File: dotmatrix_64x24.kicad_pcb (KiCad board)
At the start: 2 copper layers, 180 x 100 mm, 750 parts, among them CON1 BARREL_JACK, P1 CONN_01X09, P2 CONN_01X09, P3 CONN_01X04, P4 CONN_01X03, P5 USB_OTG, P6 CONN_01X03, Q1 NJL7302L-F3, Q2 Q_PNP_BEC 2SA1162, Q3 Q_NPN_BCE RN5006, SW1 SW_PUSH_SMALL_H, SW2 SW_PUSH_SMALL_H, SW3 SW_PUSH_SMALL_H, SW4 SW_PUSH_SMALL_H, SW5 SW_PUSH_SMALL_H, SW6 SW_PUSH_SMALL_H, SW7 SW_PUSH_SMALL_H, SW8 SW_PUSH_SMALL_H, U1 WROOM-02, U10 LED1642GW, U11 LED1642GW, U12 AE-BME280, U13 OKL-T/6-W5, U14 NJU7223, U15 DS1307, U16 CH340G, U17 OSRB38C9AA, U18 BME280, U2 74HC595-alt-vdd, U3 TD62783, U4 74HC595-alt-vdd, U5 TD62783, U6 LED1642GW, U7 74HC595-alt-vdd, U8 TD62783, U9 LED1642GW, X1 CRYSTAL_SMD, Y1 12MHz

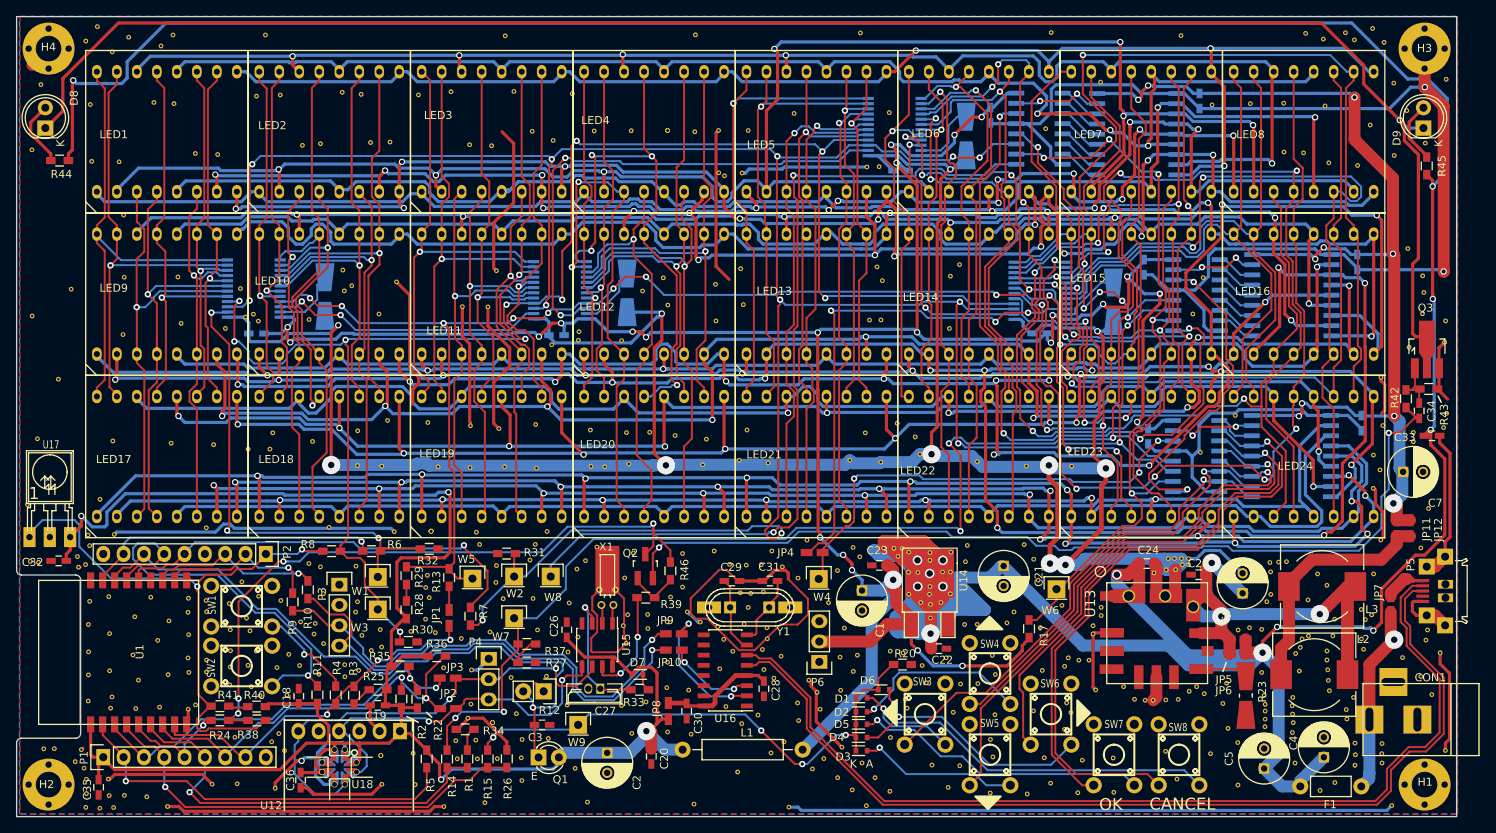
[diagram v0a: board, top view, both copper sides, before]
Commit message: Various fixes
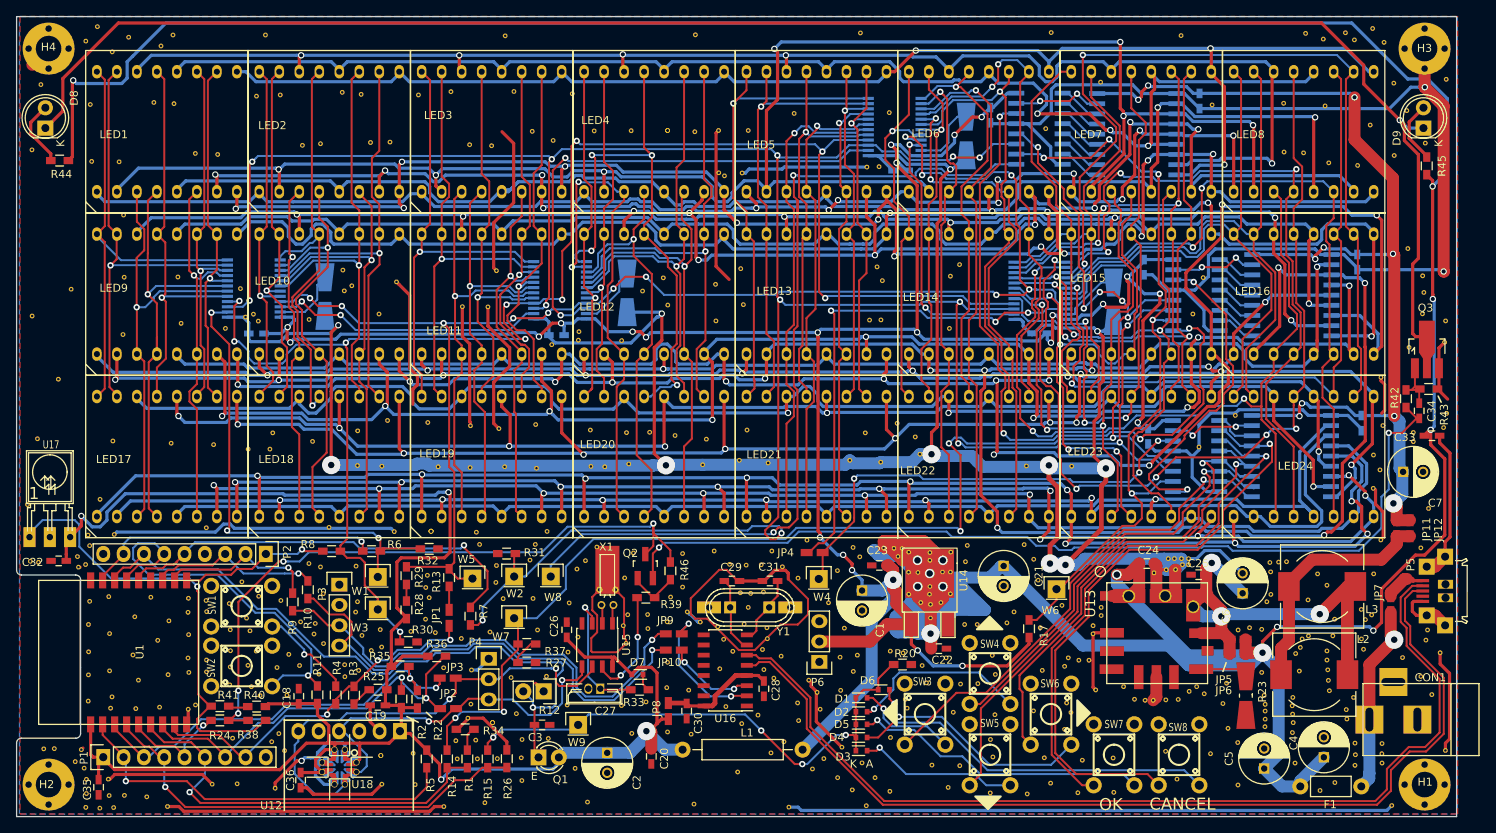
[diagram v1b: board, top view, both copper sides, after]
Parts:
- removed the REF** at (132.1, 67.6)
- removed the REF** at (166.2, 22.9)
- moved REF** 0.69 mm to (159.8, 65.8)
- moved REF** 0.32 mm to (39.0, 102.2)
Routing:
- net /Sheet57A04605/c61: track 95.8 -> 86.1 mm
- net /Sheet57A04605/SEL4: track 63.5 -> 57.2 mm
- net /Sheet57A04605/SEL5: track 71.3 -> 66.9 mm
- net /Sheet57A04605/r3: track 202.6 -> 198.6 mm
- net /Sheet57A04605/SEL6: track 80.6 -> 76.8 mm
- net /Sheet57A04605/c57: track 114.5 -> 111.2 mm
- net /Sheet57A04605/SEL3: track 70.1 -> 67.2 mm
- net /Sheet57A04605/c58: track 103.1 -> 101.9 mm
- net /Sheet57A04605/r9: track 185.2 -> 186.3 mm
- net /Sheet57A04605/r6: track 198.4 -> 199.4 mm
- net /Sheet57A04605/COLLATCH: track 203.4 -> 202.7 mm
- net /Sheet57A04605/c24: track 58.2 -> 57.5 mm
- net /Sheet57A04605/c44: track 62.7 -> 62.0 mm, vias 3 -> 2
- net Net-(P2-Pad1): track 19.5 -> 19.0 mm
- net /Sheet57A04605/c25: track 71.5 -> 70.9 mm
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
